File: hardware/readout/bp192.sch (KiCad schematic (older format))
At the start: 2 parts

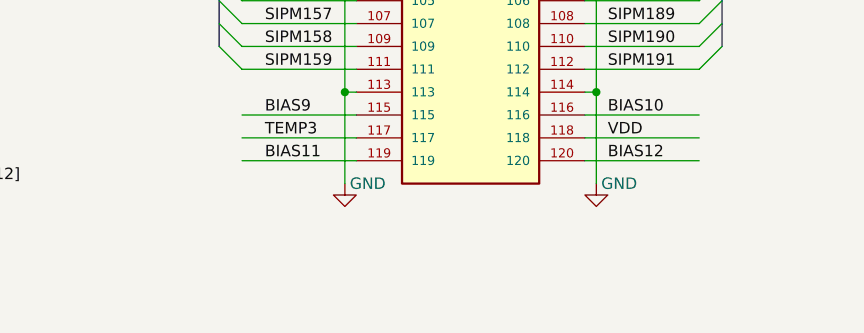
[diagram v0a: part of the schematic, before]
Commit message: schematic in progress
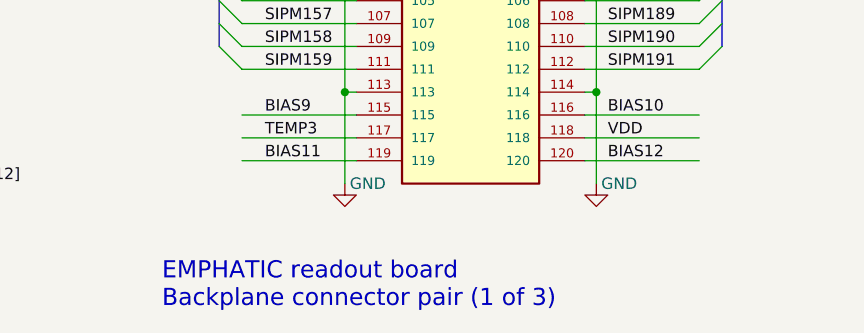
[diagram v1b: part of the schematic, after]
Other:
- note added: "EMPHATIC readout board\nBackplane connector pair (1 of 3)"
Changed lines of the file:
@@
 $Descr User 11000 9000
 encoding utf-8
-Sheet 2 35
+Sheet 2 38
 Title ""
 Date ""
@@
 Wire Bus Line
 	2650 750  2650 4350
+Text Notes 6450 7600 0    75   ~ 0
+EMPHATIC readout board\nBackplane connector pair (1 of 3)
 $EndSCHEMATC
